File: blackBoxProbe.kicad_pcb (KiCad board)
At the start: 4 copper layers, 44 x 44 mm, 80 parts, among them J1 USB-ID, J2 JTAG_2X05, J3 JTAG_2X05, J4 Conn_01x04, Q1 Q_NMOS_DUAL, Q2 Q_PMOS_DUAL, U1 MCP1702-MB, U2 USBLC6-2, U3 STM32F103CBT, U4 74X2T45, U5 74X2T45, U6 74X2T45, U7 74X2T45, Y1 8.000MHz

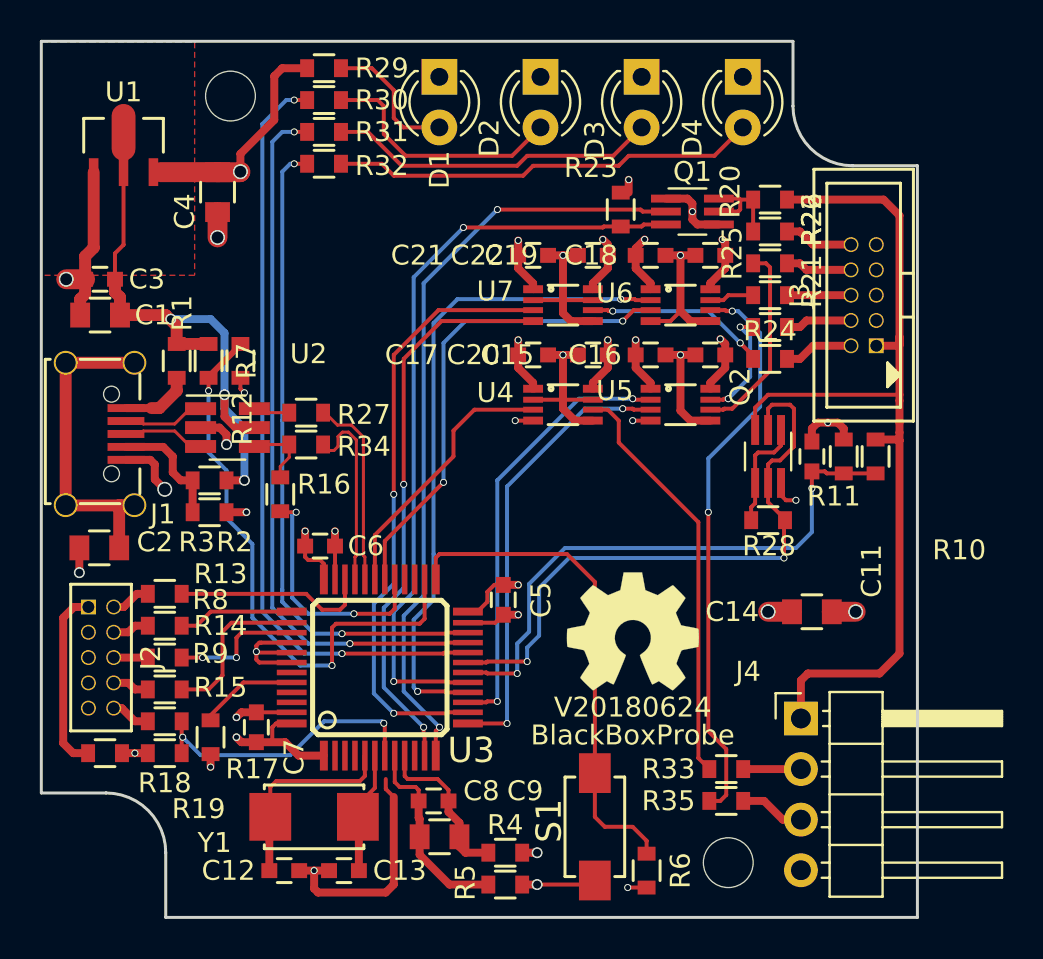
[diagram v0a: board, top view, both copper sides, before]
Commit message: WIP: final placement of silk, need some checks
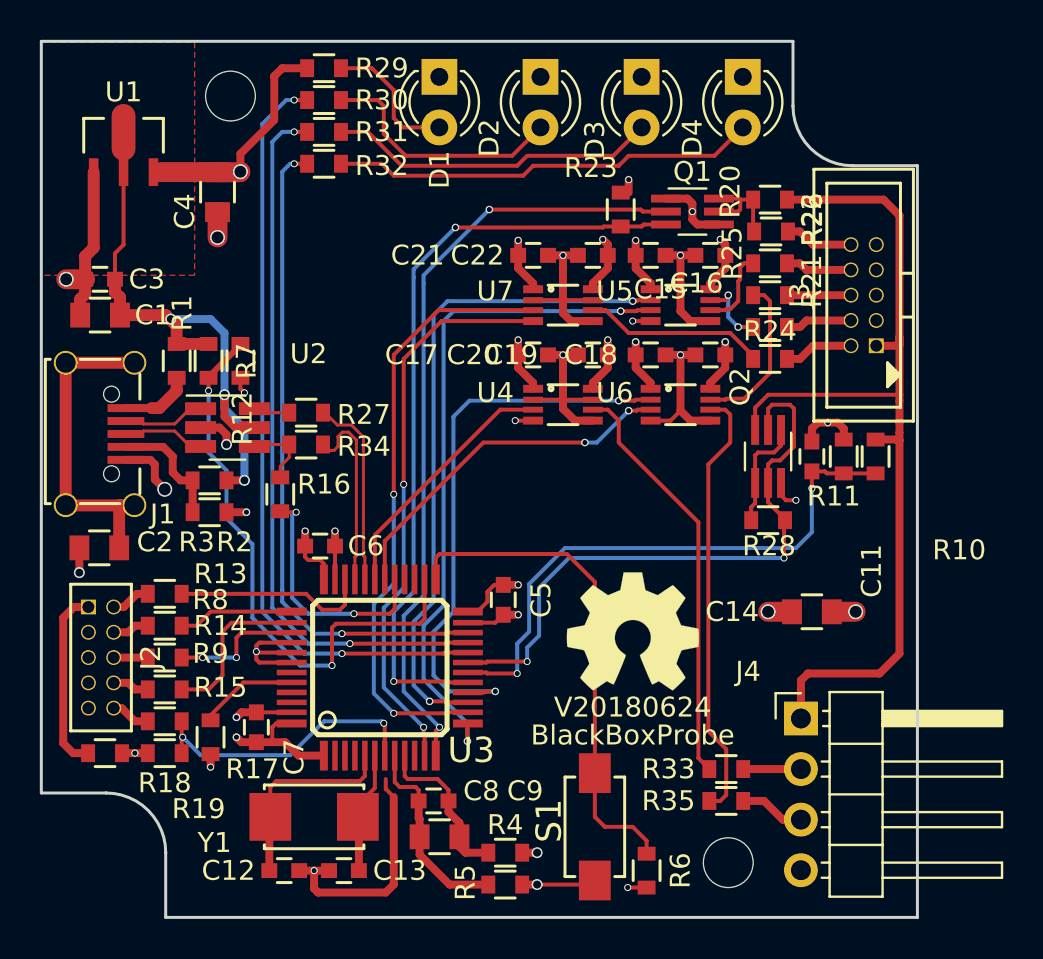
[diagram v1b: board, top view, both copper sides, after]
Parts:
- moved C15 5.00 mm to (44.9, 162.0)
- moved C16 5.00 mm to (47.9, 162.0)
- moved C18 5.00 mm to (47.9, 167.0)
- moved C19 5.00 mm to (44.9, 167.0)
- moved U5 5.00 mm to (46.4, 164.5)
- moved U6 5.00 mm to (46.4, 169.5)
- moved R26 0.05 mm to (51.0, 160.8)
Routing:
- net /PROBE_I_TCK: track 22.0 -> 33.3 mm
- net /PROBE_I_TDI: track 22.7 -> 34.0 mm
- net /PROBE_E_RX: track 28.6 -> 22.0 mm, vias 2 -> 0
- net /PROBE_I_RX: track 24.2 -> 18.0 mm
- net /PROBE_E_TDI: track 10.1 -> 4.21 mm
- net /PROBE_E_TDO: track 2.25 -> 8.13 mm
- net /PROBE_I_TDO: track 33.0 -> 28.5 mm
- net /PROBE_E_TCK: track 5.83 -> 3.62 mm
- net /PROBE_I_TX: track 13.5 -> 12.8 mm
- net /PROBE_VDD: track 86.4 -> 86.9 mm
- net /PROBE_E_TMS: vias 2 -> 0
